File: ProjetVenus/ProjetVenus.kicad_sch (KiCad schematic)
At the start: 48 parts, among them J1 Conn_01x02_Pin, J2 Conn_01x04_Pin, J4 Conn_01x02_Pin, J5 Conn_01x05_Pin, Q1 Q_NMOS_GSD, U1 ATtiny412-SS, U2 ADP2108AUJZ-3.0-R7, U3 MS5607-02BA

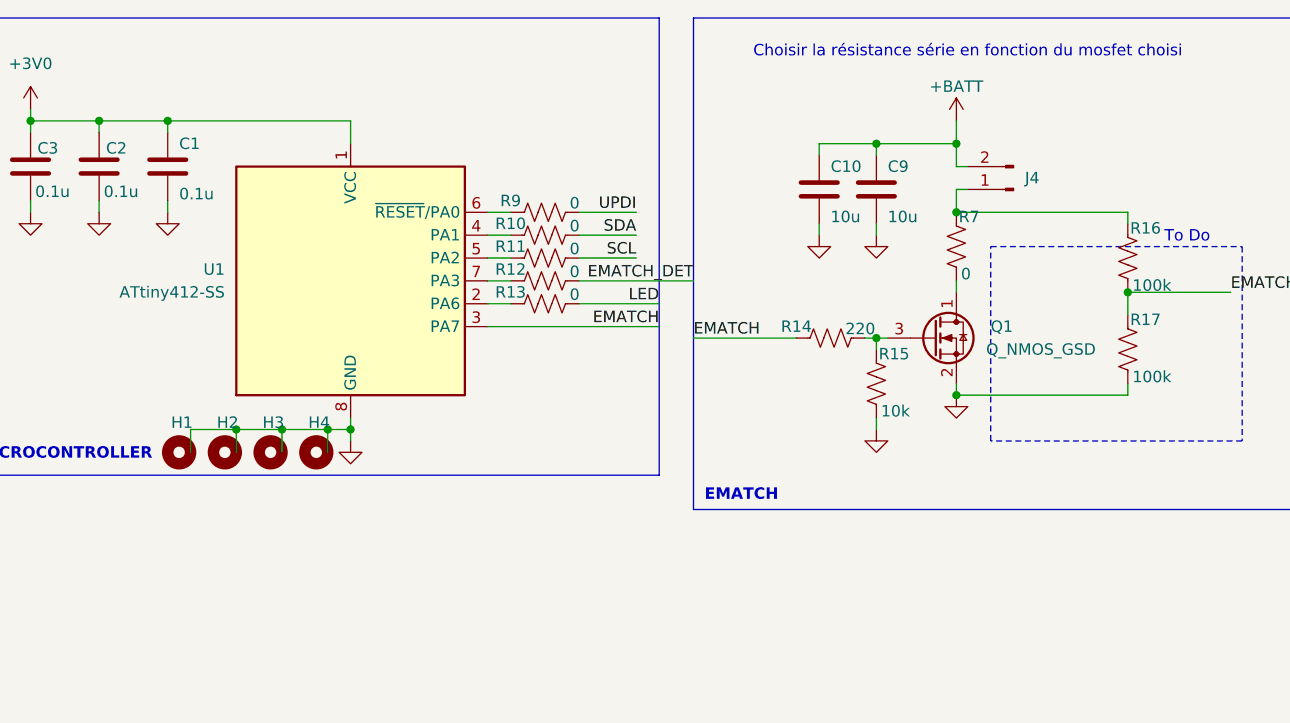
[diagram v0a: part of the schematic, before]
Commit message: V1.2
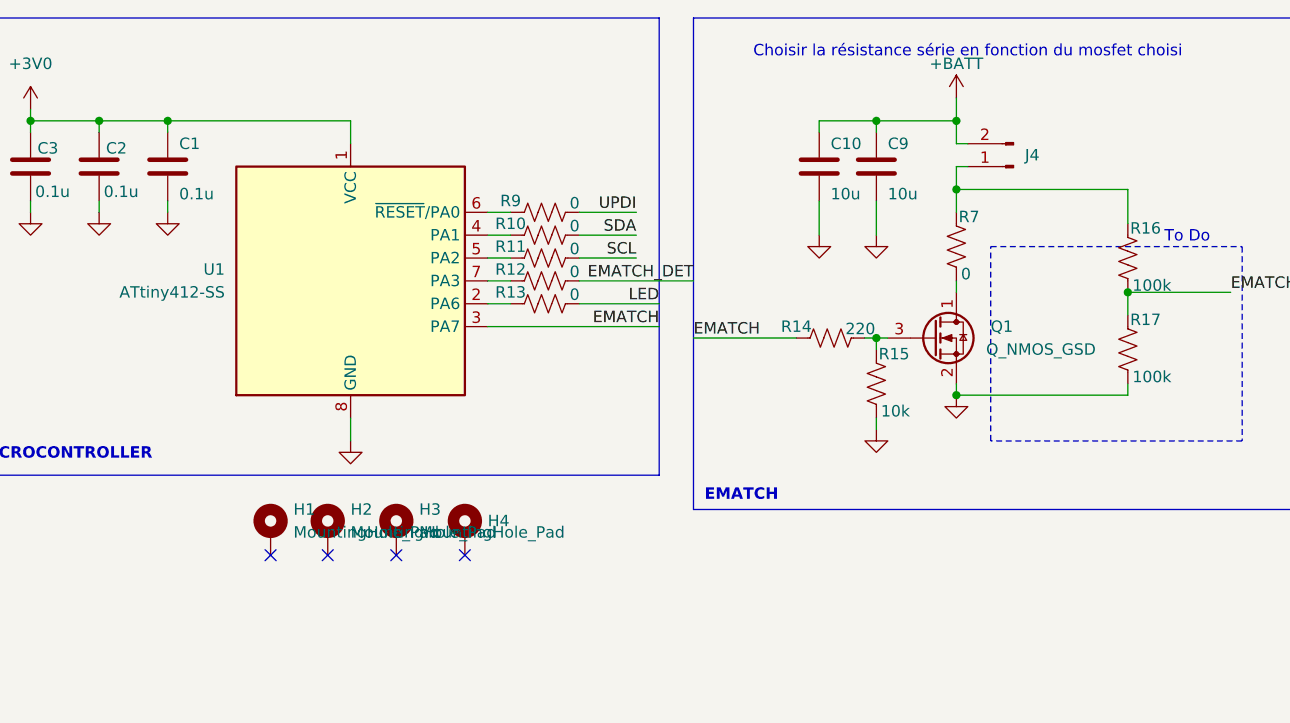
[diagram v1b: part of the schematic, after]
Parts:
- removed H1, H2, H3, H4: MountingHole, MountingHole:MountingHole_3.2mm_M3_Pad_Via, symbol Mechanical:MountingHole
- added H1, H2, H3, H4: MountingHole_Pad, MountingHole:MountingHole_3.2mm_M3_DIN965_Pad, symbol Mechanical:MountingHole_Pad
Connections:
- no-connect marks 3 -> 7
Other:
- moved on the sheet: C10, C9, J4
